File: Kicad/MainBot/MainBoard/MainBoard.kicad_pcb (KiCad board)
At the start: 4 copper layers, 158 x 134 mm, 104 parts, among them J1 Conn_01x04, J10 Conn_01x04, J11 Conn_01x04, J12 Conn_01x04, J13 01x02_DAC, J14 01x02, J15 Conn_01x24, J16 Conn_01x24, J17 01x24, J18 01x24, J19 01x05, J2 Conn_01x04, J20 01x03, J21 Conn_01x03, J22 Conn_01x03, J23 01x04, J24 01x03, J25 Conn_01x04, J26 01x04, J28 Conn_02x03_Counter_Clockwise, J29 Conn_02x03_Counter_Clockwise, J3 Conn_01x04, J30 Conn_02x03_Counter_Clockwise, J31 Conn_02x03_Counter_Clockwise, J32 Conn_01x03, J33 Conn_01x03, J34 Conn_01x02, J35 Conn_01x02, J36 Conn_01x02, J37 Conn_01x02, J38 Conn_01x03, J39 Conn_01x04, J4 Conn_01x04, J40 Conn_01x03, J41 01x04, J42 01x04, J43 01x04, J44 01x04, J5 02x04_I2C, J6 02x03, J7 02x03, J8 Conn_01x04, J9 Conn_01x04, Q1 Q_PMOS_DGS, U1 TCA9548A, U2 ISL85410, U3 Teensy3.6, U4 DRV8825, U5 DRV8825, U6 DRV8825, U7 DRV8825

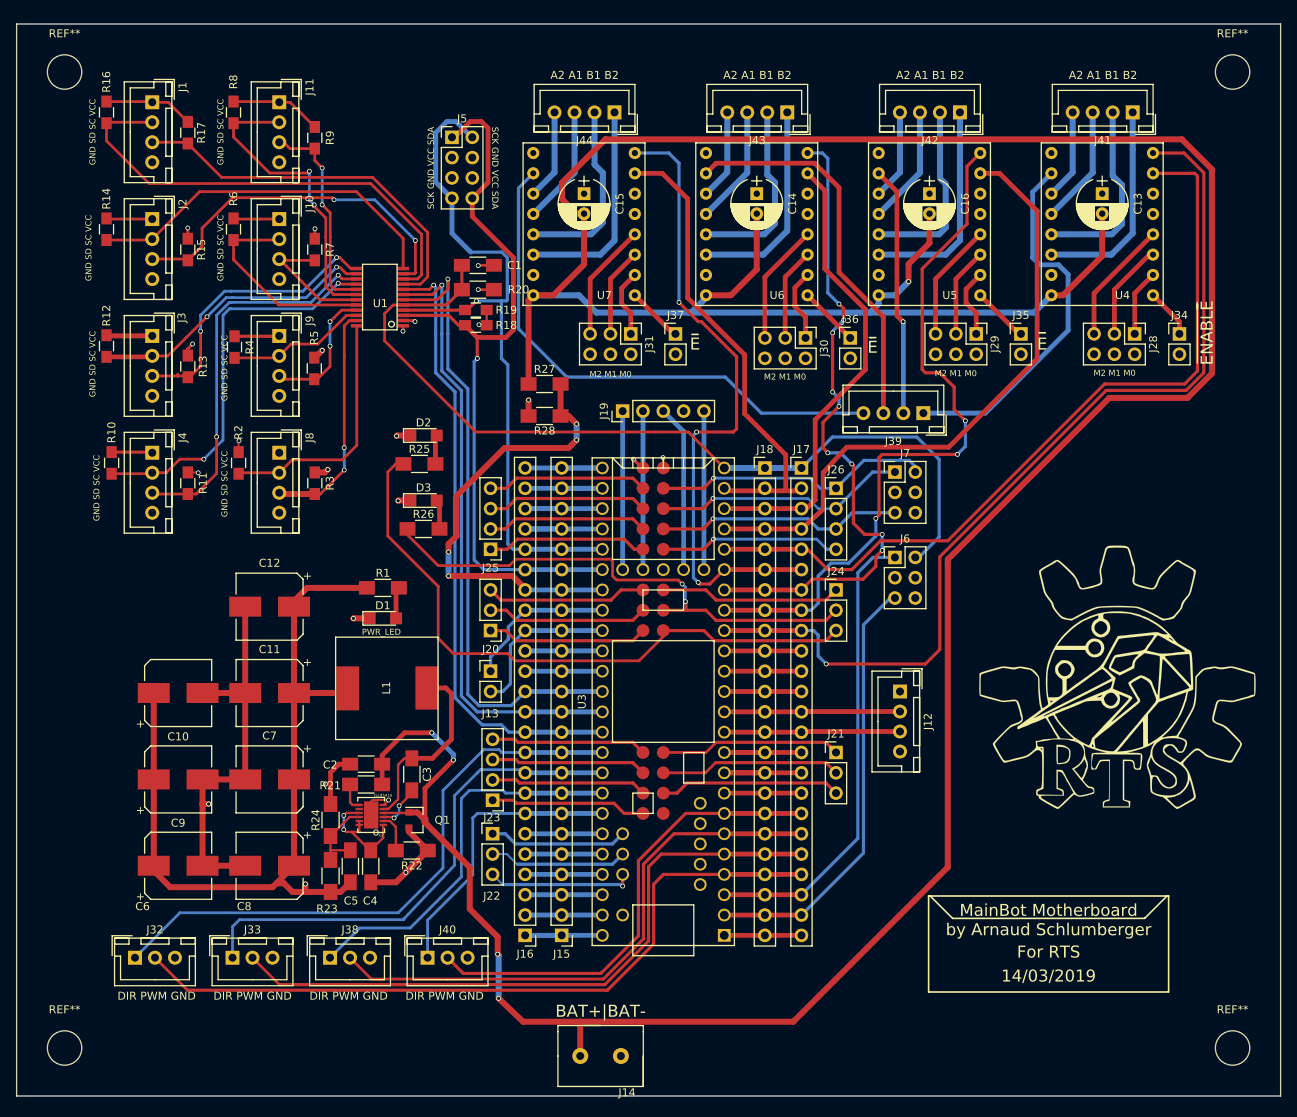
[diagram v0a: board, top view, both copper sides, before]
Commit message: ?
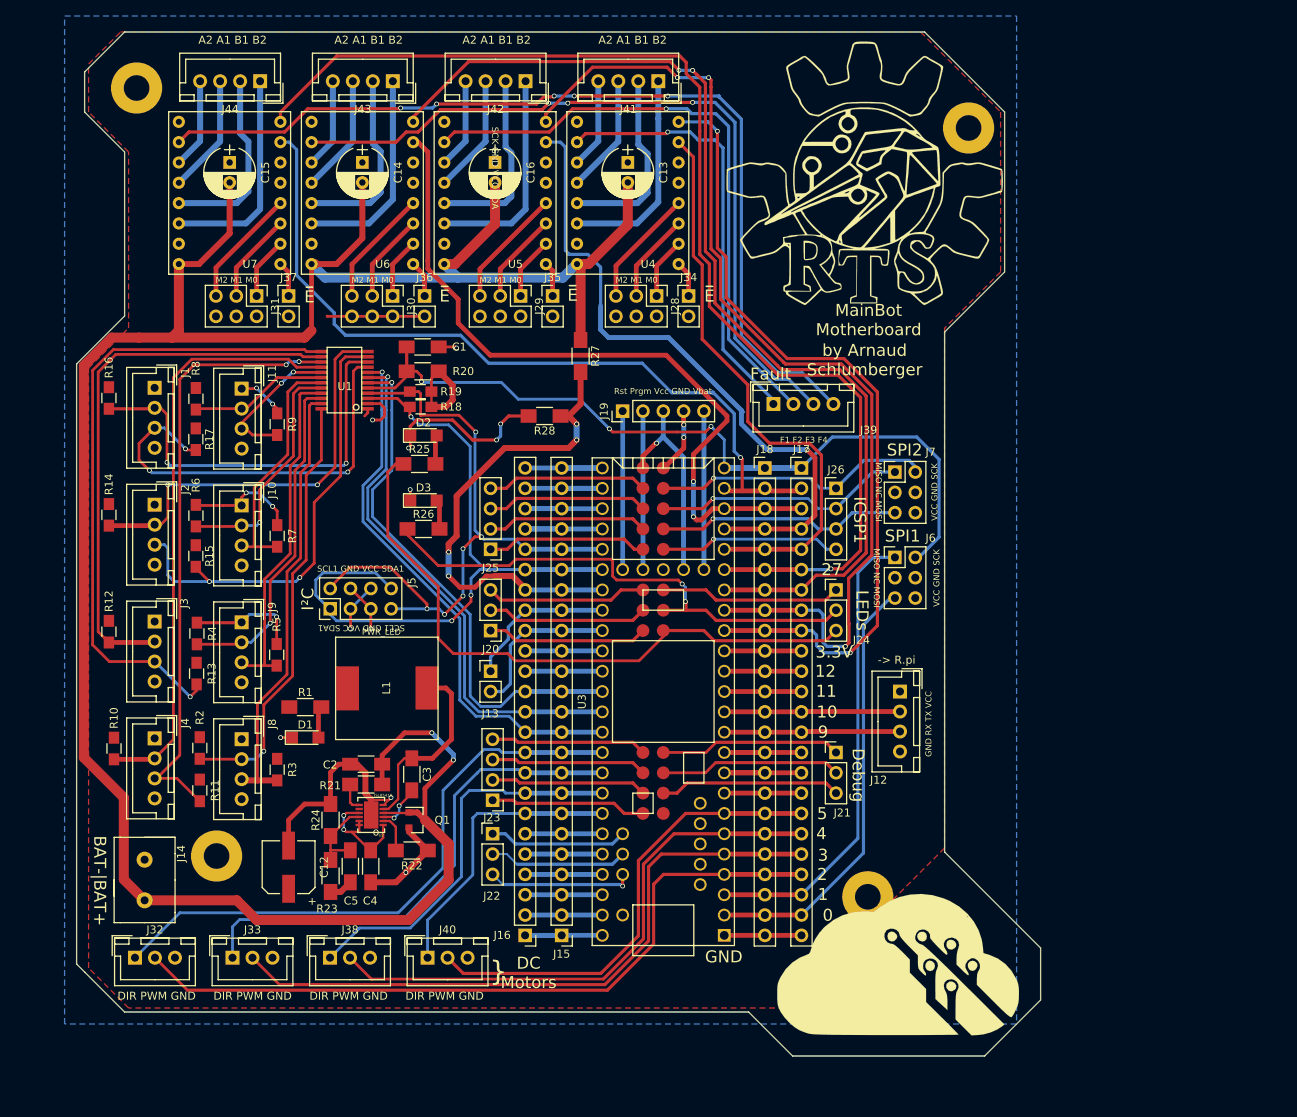
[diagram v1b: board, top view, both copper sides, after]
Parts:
- removed C10, C11, C6, C7, C8, C9: 10µF, Capacitors_SMD:CP_Elec_8x5.4
- removed REF** (x4): MountingHole_4.3mm_M4_ISO7380, Mounting_Holes:MountingHole_4.3mm_M4_ISO7380
- added ?: MountingHole_3.2mm_M3_Pad, Mounting_Holes:MountingHole_3.2mm_M3_Pad, F.Cu at (125.4, 138.1)
- added ?: MountingHole_3.2mm_M3_Pad, Mounting_Holes:MountingHole_3.2mm_M3_Pad, F.Cu at (44.0, 133.0)
- added ?: MountingHole_3.2mm_M3_Pad, Mounting_Holes:MountingHole_3.2mm_M3_Pad, F.Cu at (34.0, 37.0)
- added ?: MountingHole_3.2mm_M3_Pad, Mounting_Holes:MountingHole_3.2mm_M3_Pad, F.Cu at (138.0, 42.0)
- added G***: LOGO, Logo:aisler, F.Cu at (129.0, 146.5)
- C12: value 10µF -> 68µF; footprint Capacitors_SMD:CP_Elec_8x5.4 -> Capacitors_SMD:CP_Elec_6.3x7.7
- moved G*** 70.5 mm to (125.0, 50.0)
- moved J34 61.5 mm to (103.0, 63.0)
- moved J14 61.1 mm to (35.0, 136.0), turned to 270 degrees
- moved J5 60.9 mm to (58.2, 102.1), turned to 90 degrees
- moved J28 60.0 mm to (99.0, 63.0)
- moved J41 59.4 mm to (99.2, 36.1)
- moved C13 59.4 mm to (95.4, 46.3)
- moved U4 59.4 mm to (95.4, 50.1)
- moved J35 58.7 mm to (86.0, 63.0)
- moved J29 57.1 mm to (82.0, 63.0)
- moved C16 54.4 mm to (78.8, 46.3)
- moved U5 54.4 mm to (78.8, 50.1)
- moved J42 54.4 mm to (82.6, 36.1)
- moved J36 53.5 mm to (70.0, 63.0)
- moved J30 51.9 mm to (66.0, 63.0)
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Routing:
- net +12C: track 464.8 -> 303.7 mm, vias 5 -> 2
- net VCC: track 234.1 -> 123.1 mm, vias 12 -> 7
- net /STEP_DIR_4: track 80.6 -> 147.9 mm, vias 3 -> 1
- net /STEP_DIR_3: track 82.2 -> 132.2 mm, vias 9 -> 2
- net /FAU_4: track 67.7 -> 116.1 mm, vias 0 -> 5
- net /FAU_3: track 48.9 -> 96.2 mm, vias 0 -> 3
- net /FAU_2: track 31.3 -> 76.3 mm
- net /M_SD2: track 36.8 -> 81.1 mm, vias 2 -> 1
- net /A12: track 62.2 -> 103.8 mm, vias 0 -> 1
- net /STEP_DIR_2: track 89.1 -> 128.4 mm
- net /PWM_11: track 58.2 -> 93.0 mm, vias 0 -> 2
- net /M_SC2: track 36.6 -> 69.4 mm, vias 2 -> 0
- net /STEP_STP_1: track 101.3 -> 72.1 mm
- net /M_SD3: track 49.0 -> 77.0 mm
- net /M_SD6: track 17.3 -> 44.2 mm, vias 2 -> 0
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- added copper zone on B.Cu, net GND
- added copper zone on F.Cu, net VCC
- removed copper zone on In2.Cu, net GND
- removed copper zone on VccPlane.Cu, net VCC
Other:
- board size 158 x 134 mm -> 120.5 x 128 mm
- copper layers 4 -> 2
- board text added: "-> R.pi"
- board text added: "0"
- board text added: "1"
- board text added: "10"
- board text added: "11"
- board text added: "12"
- board text added: "2"
- board text added: "27"
- board text added: "3"
- board text added: "3.3V"
- board text added: "4"
- board text added: "5"
- board text added: "9"
- board text added: "BAT-|BAT+"
- board text added: "DC Motors"
- board text added: "Debug"
- board text added: "F1 F2 F3 F4"
- board text added: "Fault"
- board text added: "GND"
- board text added: "GND RX TX VCC"
- board text added: "ICSP1"
- board text added: "I²C"
- board text added: "LEDs"
- board text added: "MISO NC MOSI"
- board text added: "MainBot Motherboard"
- board text added: "Rst Prgm Vcc GND Vbat"
- board text added: "SCL1 GND VCC SDA1"
- board text added: "SPI1"
- board text added: "SPI2"
- board text added: "VCC GND SCK"
- board text added: "by Arnaud Schlumberger"
- board text added: "}"
- board text removed: "14/03/2019"
- board text removed: "BAT+|BAT-"
- board text removed: "ENABLE"
- board text removed: "For RTS"
- board text removed: "GND SD SC VCC"
- board text removed: "MainBot Motherboard by Arnaud Schlumberger"
